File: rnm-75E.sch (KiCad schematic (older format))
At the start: 12 parts

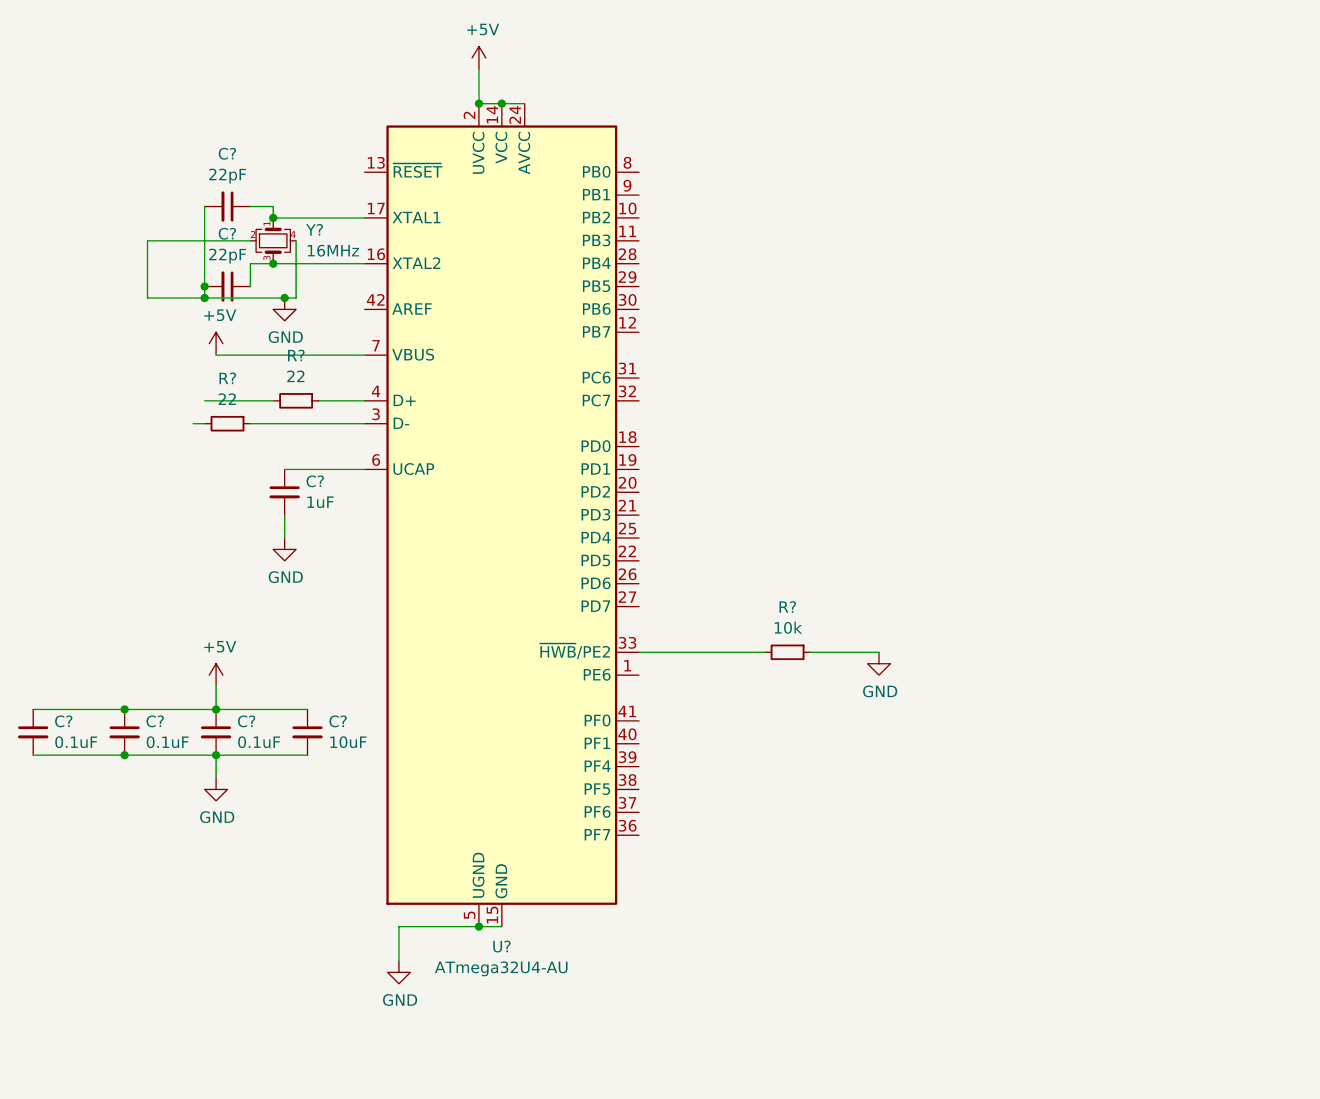
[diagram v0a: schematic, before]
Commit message: new crystal
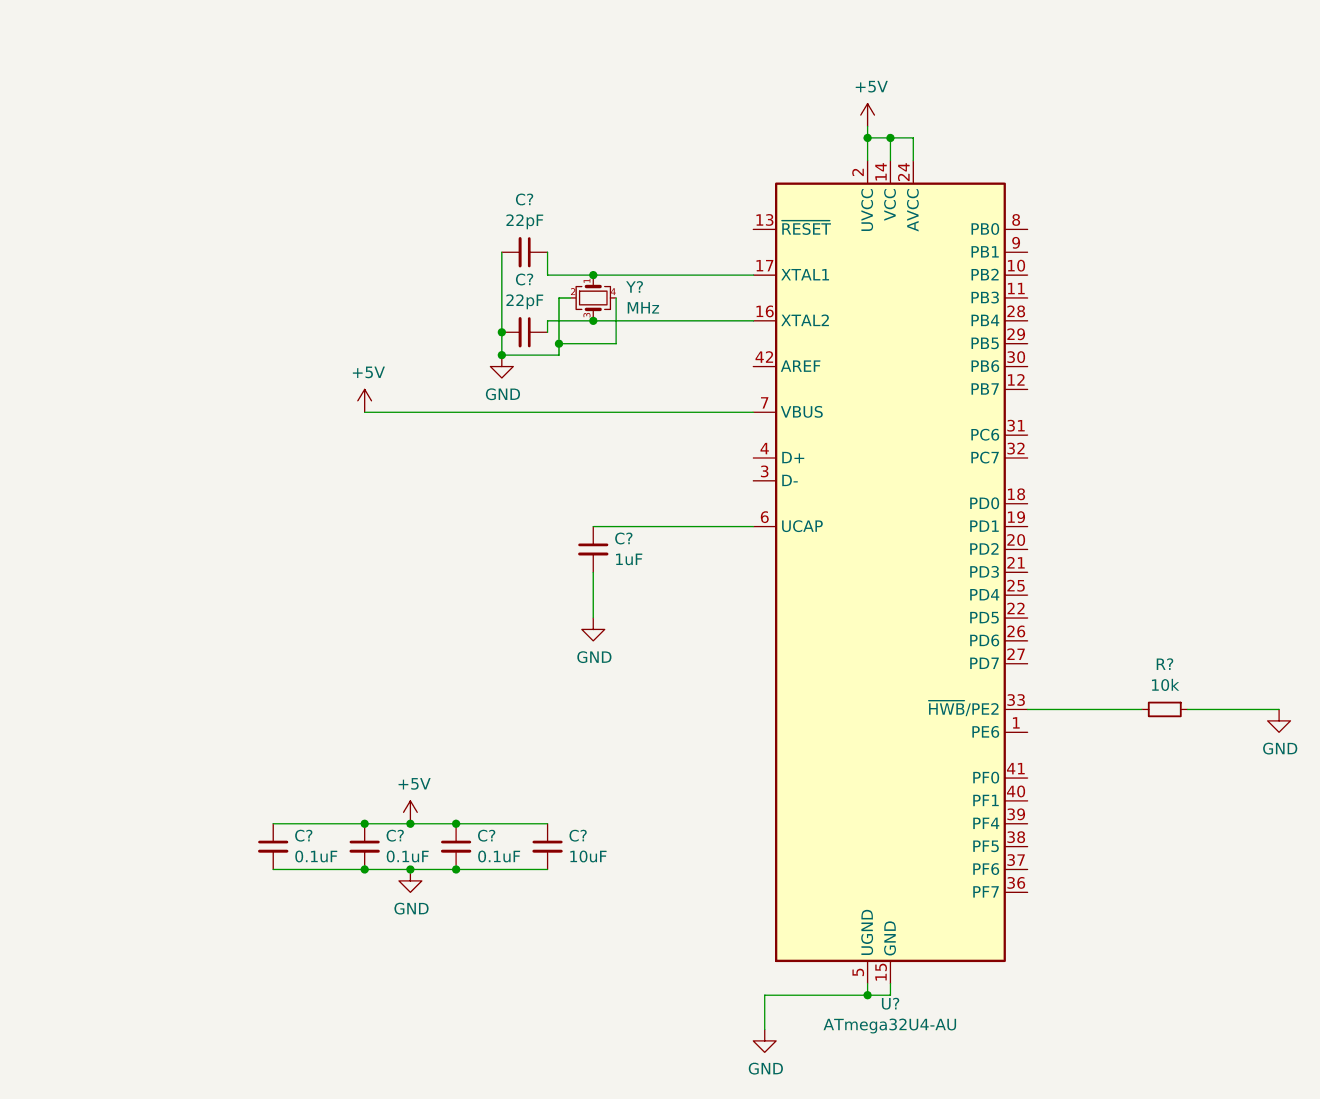
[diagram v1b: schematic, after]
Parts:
- removed C?: 1uF, symbol Device:C_Small
- removed C? (x3): 0.1uF, symbol Device:C_Small
- removed C?: 10uF, symbol Device:C_Small
- removed C? (x2): 22pF, symbol Device:C_Small
- removed R?: 10k, symbol Device:R_Small
- removed R? (x2): 22, symbol Device:R_Small
- removed U?: ATmega32U4-AU, Package_QFP:TQFP-44_10x10mm_P0.8mm, symbol MCU_Microchip_ATmega:ATmega32U4-AU
- removed Y?: 16MHz, symbol Device:Crystal_GND24_Small
- added C?: 1uF, symbol Device:C_Small
- added C? (x3): 0.1uF, symbol Device:C_Small
- added C?: 10uF, symbol Device:C_Small
- added C? (x2): 22pF, symbol Device:C_Small
- added R?: 10k, symbol Device:R_Small
- added U?: ATmega32U4-AU, Package_QFP:TQFP-44_10x10mm_P0.8mm, symbol MCU_Microchip_ATmega:ATmega32U4-AU
- added Y?: MHz, symbol Device:Crystal_GND24_Small
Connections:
- wire segments 37 -> 38
